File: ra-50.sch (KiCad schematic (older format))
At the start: 172 parts, among them J1 Conn_01x07, J2 Conn_01x05, J3 Conn_01x05, J4 Conn_01x12, J5 Conn_01x20, SW1 MX-NoLED, SW10 MX-NoLED, SW11 MX-NoLED, SW12 MX-NoLED, SW13 MX-NoLED, SW14 MX-NoLED, SW14B1 Rotary_Encoder_Switch, SW15 MX-NoLED, SW16 MX-NoLED, SW17 MX-NoLED, SW18 MX-NoLED, SW19 MX-NoLED, SW2 MX-NoLED, SW20 MX-NoLED, SW21 MX-NoLED, SW22 MX-NoLED, SW23 MX-NoLED, SW24 MX-NoLED, SW25 MX-NoLED, SW26 MX-NoLED, SW27 MX-NoLED, SW28 MX-NoLED, SW29 MX-NoLED, SW3 MX-NoLED, SW30 MX-NoLED, SW31 MX-NoLED, SW32 MX-NoLED, SW33 MX-NoLED, SW34 MX-NoLED, SW35 MX-NoLED, SW36 MX-NoLED, SW37 MX-NoLED, SW38 MX-NoLED, SW39 MX-NoLED, SW4 MX-NoLED, SW40 MX-NoLED, SW41 MX-NoLED, SW42 MX-NoLED, SW43 MX-NoLED, SW44 MX-NoLED, SW45 MX-NoLED, SW46 MX-NoLED, SW47 MX-NoLED, SW48 MX-NoLED, SW49 MX-NoLED, SW5 MX-NoLED, SW50 MX-NoLED, SW51 MX-NoLED, SW52 MX-NoLED, SW53 MX-NoLED, SW54 MX-NoLED, SW55 MX-NoLED, SW56 MX-NoLED, SW57 MX-NoLED, SW58 MX-NoLED, SW59 MX-NoLED, SW6 MX-NoLED, SW60 MX-NoLED, SW61 MX-NoLED, SW62 MX-NoLED, SW63 MX-NoLED, SW64 MX-NoLED, SW65 MX-NoLED, SW66 MX-NoLED, SW67 MX-NoLED, SW68 MX-NoLED, SW69 MX-NoLED, SW7 MX-NoLED, SW8 MX-NoLED, SW9 MX-NoLED

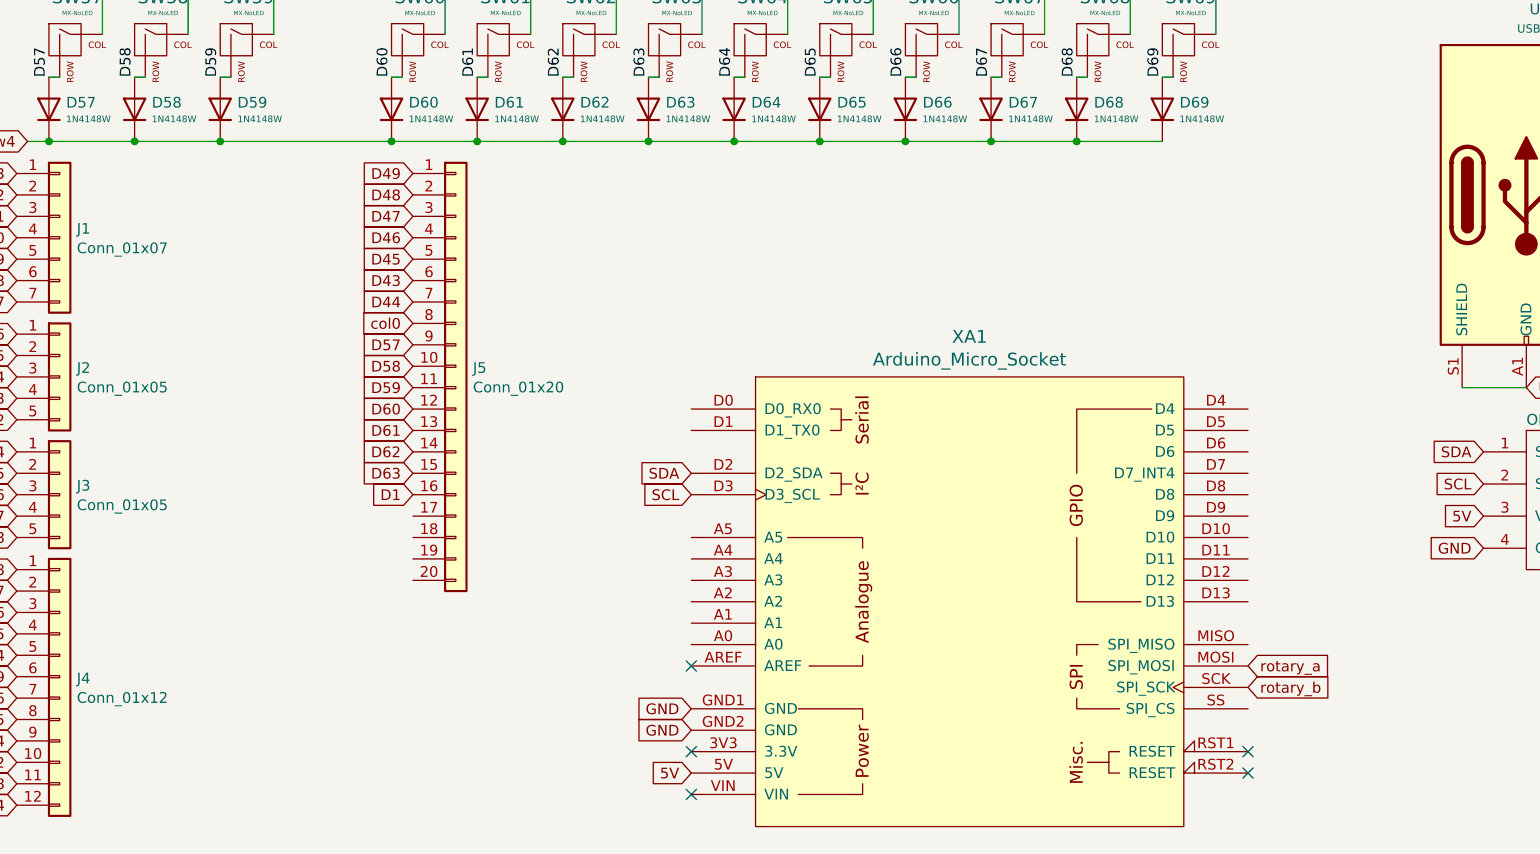
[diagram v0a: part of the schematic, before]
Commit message: update
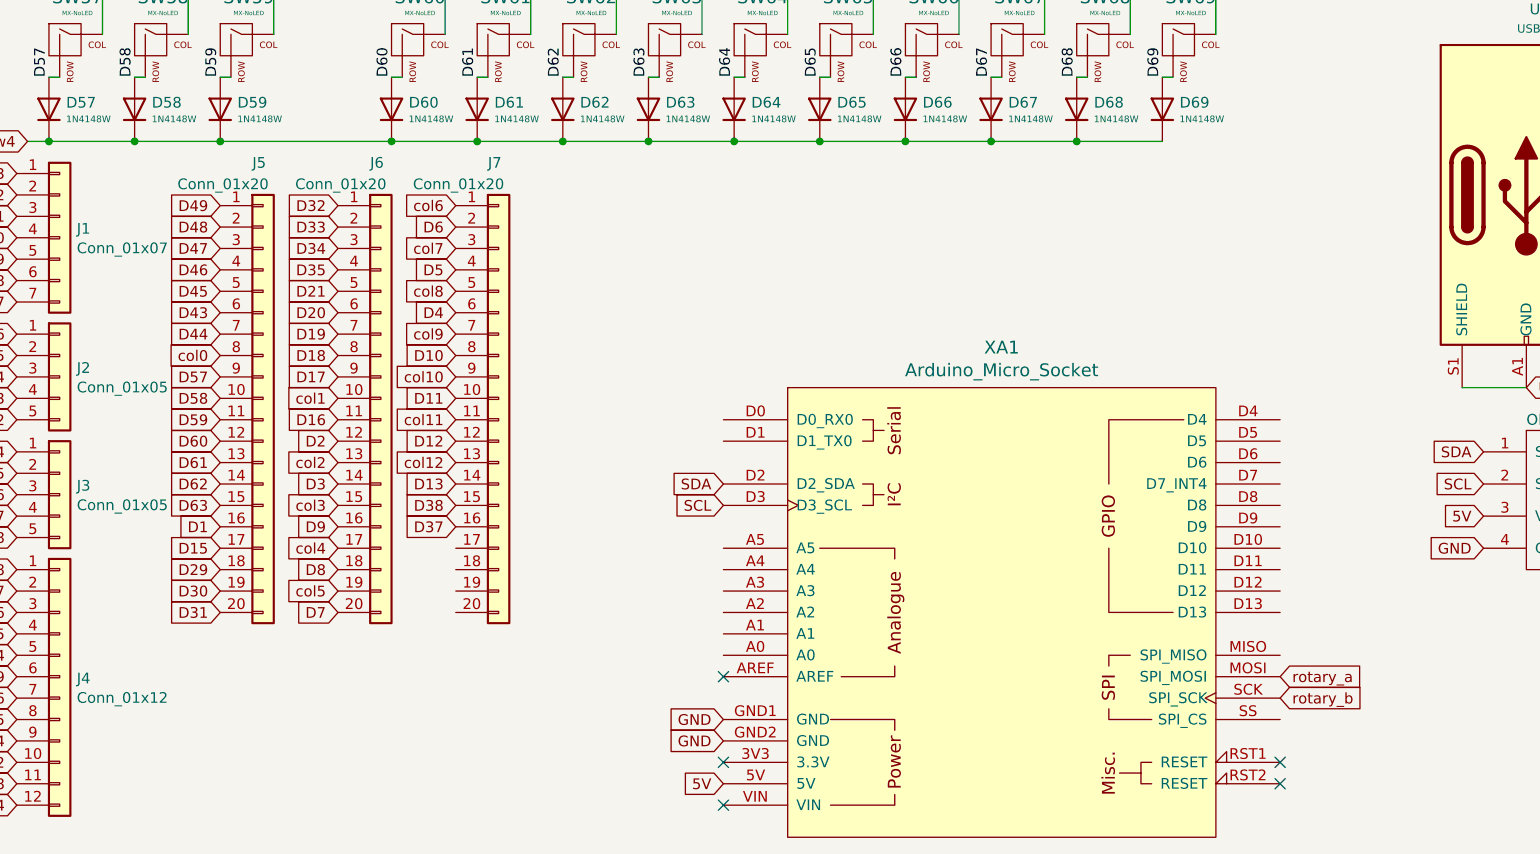
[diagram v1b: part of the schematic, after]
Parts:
- added J6, J7: Conn_01x20, locallib:PinHeader_1x20_via, symbol Connector_Generic:Conn_01x20
- J5: footprint Connector_PinHeader_1.00mm:PinHeader_1x20_P1.00mm_Vertical -> locallib:PinHeader_1x20_via
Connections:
- net D10: now also J7.8 (Pin_8)
- net D11: now also J7.10 (Pin_10)
- net D12: now also J7.12 (Pin_12)
- net D13: now also J7.14 (Pin_14)
- net D15: now also J5.17 (Pin_17)
- net D16: now also J6.11 (Pin_11)
- net D17: now also J6.9 (Pin_9)
- net D18: now also J6.8 (Pin_8)
- net D19: now also J6.7 (Pin_7)
- net D2: now also J6.12 (Pin_12)
- net D20: now also J6.6 (Pin_6)
- net D21: now also J6.5 (Pin_5)
- net D29: now also J5.18 (Pin_18)
- net D3: now also J6.14 (Pin_14)
- net D30: now also J5.19 (Pin_19)
- net D31: now also J5.20 (Pin_20)
- net D32: now also J6.1 (Pin_1)
- net D33: now also J6.2 (Pin_2)
- net D34: now also J6.3 (Pin_3)
- net D35: now also J6.4 (Pin_4)
- net D37: now also J7.16 (Pin_16)
- net D38: now also J7.15 (Pin_15)
- net D4: now also J7.6 (Pin_6)
- net D5: now also J7.4 (Pin_4)
- net D6: now also J7.2 (Pin_2)
- net D7: now also J6.20 (Pin_20)
- net D8: now also J6.18 (Pin_18)
- net D9: now also J6.16 (Pin_16)
- net col1: now also J6.10 (Pin_10)
- net col10: now also J7.9 (Pin_9)
- net col11: now also J7.11 (Pin_11)
- net col12: now also J7.13 (Pin_13)
- net col2: now also J6.13 (Pin_13)
- net col3: now also J6.15 (Pin_15)
- net col4: now also J6.17 (Pin_17)
- net col5: now also J6.19 (Pin_19)
- net col6: now also J7.1 (Pin_1)
- net col7: now also J7.3 (Pin_3)
- net col8: now also J7.5 (Pin_5)
- net col9: now also J7.7 (Pin_7)
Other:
- moved on the sheet: J5, XA1
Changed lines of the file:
@@
 L arduino:Arduino_Micro_Socket XA1
 U 1 1 60EDE630
-P 5150 6650
-F 0 "XA1" H 5150 7887 60  0000 C CNN
-F 1 "Arduino_Micro_Socket" H 5150 7781 60  0000 C CNN
-F 2 "Arduino:Arduino_Micro_Socket" H 6950 10400 60  0001 C CNN
-F 3 "https://store.arduino.cc/arduino-micro" H 6950 10400 60  0001 C CNN
-	1    5150 6650
-	1    0    0    -1
-$EndComp
-Text GLabel 3850 7450 0    50   Input ~ 0
+P 5300 6700
+F 0 "XA1" H 5300 7937 60  0000 C CNN
+F 1 "Arduino_Micro_Socket" H 5300 7831 60  0000 C CNN
+F 2 "Arduino:Arduino_Micro_Socket" H 7100 10450 60  0001 C CNN
+F 3 "https://store.arduino.cc/arduino-micro" H 7100 10450 60  0001 C CNN
+	1    5300 6700
+	1    0    0    -1
+$EndComp
+Text GLabel 4000 7500 0    50   Input ~ 0
 5V
-Text GLabel 3850 7250 0    50   Input ~ 0
+Text GLabel 4000 7300 0    50   Input ~ 0
 GND
-NoConn ~ 3850 7350
-NoConn ~ 3850 7550
-NoConn ~ 3850 6950
-NoConn ~ 6450 7350
-NoConn ~ 6450 7450
+NoConn ~ 4000 7400
+NoConn ~ 4000 7600
+NoConn ~ 4000 7000
+NoConn ~ 6600 7400
+NoConn ~ 6600 7500
 Text GLabel 7550 5950 0    50   Input ~ 0
 SDA
@@
 	-1   0    0    1
 $EndComp
-Text GLabel 3850 7150 0    50   Input ~ 0
+Text GLabel 4000 7200 0    50   Input ~ 0
 GND
 Text GLabel 7250 1200 2    50   Input ~ 0
 GND
-Text GLabel 3850 6150 0    50   Input ~ 0
+Text GLabel 4000 6200 0    50   Input ~ 0
 SCL
-Text GLabel 3850 6050 0    50   Input ~ 0
+Text GLabel 4000 6100 0    50   Input ~ 0
 SDA
-Text GLabel 6450 7050 2    50   Input ~ 0
+Text GLabel 6600 7100 2    50   Input ~ 0
 rotary_b
-Text GLabel 6450 6950 2    50   Input ~ 0
+Text GLabel 6600 7000 2    50   Input ~ 0
 rotary_a
 $Comp
@@
 L Connector_Generic:Conn_01x20 J5
 U 1 1 612D088F
-P 2750 5550
-F 0 "J5" H 2830 5542 50  0000 L CNN
-F 1 "Conn_01x20" H 2830 5451 50  0000 L CNN
-F 2 "Connector_PinHeader_1.00mm:PinHeader_1x20_P1.00mm_Vertical" H 2750 5550 50  0001 C CNN
-F 3 "~" H 2750 5550 50  0001 C CNN
-	1    2750 5550
+P 1850 5700
+F 0 "J5" H 1800 6800 50  0000 L CNN
+F 1 "Conn_01x20" H 1450 6700 50  0000 L CNN
+F 2 "locallib:PinHeader_1x20_via" H 1850 5700 50  0001 C CNN
+F 3 "~" H 1850 5700 50  0001 C CNN
+	1    1850 5700
 	1    0    0    -1
 $EndComp
@@
 Text Label 5650 2700 1    50   ~ 0
 D41
-Text GLabel 2550 4650 0    50   Input ~ 0
+Text GLabel 1650 4800 0    50   Input ~ 0
 D49
-Text GLabel 2550 4750 0    50   Input ~ 0
+Text GLabel 1650 4900 0    50   Input ~ 0
 D48
-Text GLabel 2550 4850 0    50   Input ~ 0
+Text GLabel 1650 5000 0    50   Input ~ 0
 D47
-Text GLabel 2550 4950 0    50   Input ~ 0
+Text GLabel 1650 5100 0    50   Input ~ 0
 D46
-Text GLabel 2550 5050 0    50   Input ~ 0
+Text GLabel 1650 5200 0    50   Input ~ 0
 D45
-Text GLabel 2550 5150 0    50   Input ~ 0
+Text GLabel 1650 5300 0    50   Input ~ 0
 D43
-Text GLabel 2550 5250 0    50   Input ~ 0
+Text GLabel 1650 5400 0    50   Input ~ 0
 D44
-Text GLabel 2550 6050 0    50   Input ~ 0
+Text GLabel 1650 6200 0    50   Input ~ 0
 D63
-Text GLabel 2550 5950 0    50   Input ~ 0
+Text GLabel 1650 6100 0    50   Input ~ 0
 D62
-Text GLabel 2550 5850 0    50   Input ~ 0
+Text GLabel 1650 6000 0    50   Input ~ 0
 D61
-Text GLabel 2550 5750 0    50   Input ~ 0
+Text GLabel 1650 5900 0    50   Input ~ 0
 D60
-Text GLabel 2550 5650 0    50   Input ~ 0
+Text GLabel 1650 5800 0    50   Input ~ 0
 D59
-Text GLabel 2550 5550 0    50   Input ~ 0
+Text GLabel 1650 5700 0    50   Input ~ 0
 D58
-Text GLabel 2550 5450 0    50   Input ~ 0
+Text GLabel 1650 5600 0    50   Input ~ 0
 D57
-Text GLabel 2550 5350 0    50   Input ~ 0
+Text GLabel 1650 5500 0    50   Input ~ 0
 col0
-Text GLabel 2550 6150 0    50   Input ~ 0
+Text GLabel 1650 6300 0    50   Input ~ 0
 D1
 $Comp
@@
 	1    0    0    -1
 $EndComp
+Text GLabel 1650 6400 0    50   Input ~ 0
+D15
+Text GLabel 1650 6500 0    50   Input ~ 0
+D29
+Text GLabel 1650 6600 0    50   Input ~ 0
+D30
+Text GLabel 2200 5700 0    50   Input ~ 0
+col1
+Text GLabel 1650 6700 0    50   Input ~ 0
+D31
+Text GLabel 2200 4800 0    50   Input ~ 0
+D32
+Text GLabel 2200 4900 0    50   Input ~ 0
+D33
+Text GLabel 2200 5000 0    50   Input ~ 0
+D34
+Text GLabel 2200 5100 0    50   Input ~ 0
+D35
+Text GLabel 2200 5200 0    50   Input ~ 0
+D21
+Text GLabel 2200 5300 0    50   Input ~ 0
+D20
+Text GLabel 2200 5400 0    50   Input ~ 0
+D19
+Text GLabel 2200 5500 0    50   Input ~ 0
+D18
+Text GLabel 2200 5600 0    50   Input ~ 0
+D17
+Text GLabel 2200 5800 0    50   Input ~ 0
+D16
+Text GLabel 2200 5900 0    50   Input ~ 0
+D2
+Text GLabel 2200 6000 0    50   Input ~ 0
+col2
+Text GLabel 2200 6100 0    50   Input ~ 0
+D3
+Text GLabel 2750 5700 0    50   Input ~ 0
+D11
+Text GLabel 2750 5900 0    50   Input ~ 0
+D12
+Text GLabel 2750 6100 0    50   Input ~ 0
+D13
+Text GLabel 2200 6200 0    50   Input ~ 0
+col3
+Text GLabel 2200 6400 0    50   Input ~ 0
+col4
+Text GLabel 2750 5500 0    50   Input ~ 0
+D10
+$Comp
+L Connector_Generic:Conn_01x20 J6
+U 1 1 60F7AB70
+P 2400 5700
+F 0 "J6" H 2350 6800 50  0000 L CNN
+F 1 "Conn_01x20" H 2000 6700 50  0000 L CNN
+F 2 "locallib:PinHeader_1x20_via" H 2400 5700 50  0001 C CNN
+F 3 "~" H 2400 5700 50  0001 C CNN
+	1    2400 5700
+	1    0    0    -1
+$EndComp
+Text GLabel 2200 6600 0    50   Input ~ 0
+col5
+Text GLabel 2750 4800 0    50   Input ~ 0
+col6
+Text GLabel 2750 5000 0    50   Input ~ 0
+col7
+Text GLabel 2750 5200 0    50   Input ~ 0
+col8
+Text GLabel 2750 5400 0    50   Input ~ 0
+col9
+Text GLabel 2750 5600 0    50   Input ~ 0
+col10
+Text GLabel 2750 5800 0    50   Input ~ 0
+col11
+Text GLabel 2750 6000 0    50   Input ~ 0
+col12
+Text GLabel 2750 6200 0    50   Input ~ 0
+D38
+Text GLabel 2200 6700 0    50   Input ~ 0
+D7
+Text GLabel 2200 6500 0    50   Input ~ 0
+D8
+Text GLabel 2750 4900 0    50   Input ~ 0
+D6
+Text GLabel 2750 5100 0    50   Input ~ 0
+D5
+Text GLabel 2750 5300 0    50   Input ~ 0
+D4
+Text GLabel 2200 6300 0    50   Input ~ 0
+D9
+$Comp
+L Connector_Generic:Conn_01x20 J7
+U 1 1 6115908E
+P 2950 5700
+F 0 "J7" H 2900 6800 50  0000 L CNN
+F 1 "Conn_01x20" H 2550 6700 50  0000 L CNN
+F 2 "locallib:PinHeader_1x20_via" H 2950 5700 50  0001 C CNN
+F 3 "~" H 2950 5700 50  0001 C CNN
+	1    2950 5700
+	1    0    0    -1
+$EndComp
+Text GLabel 2750 6300 0    50   Input ~ 0
+D37
 $EndSCHEMATC

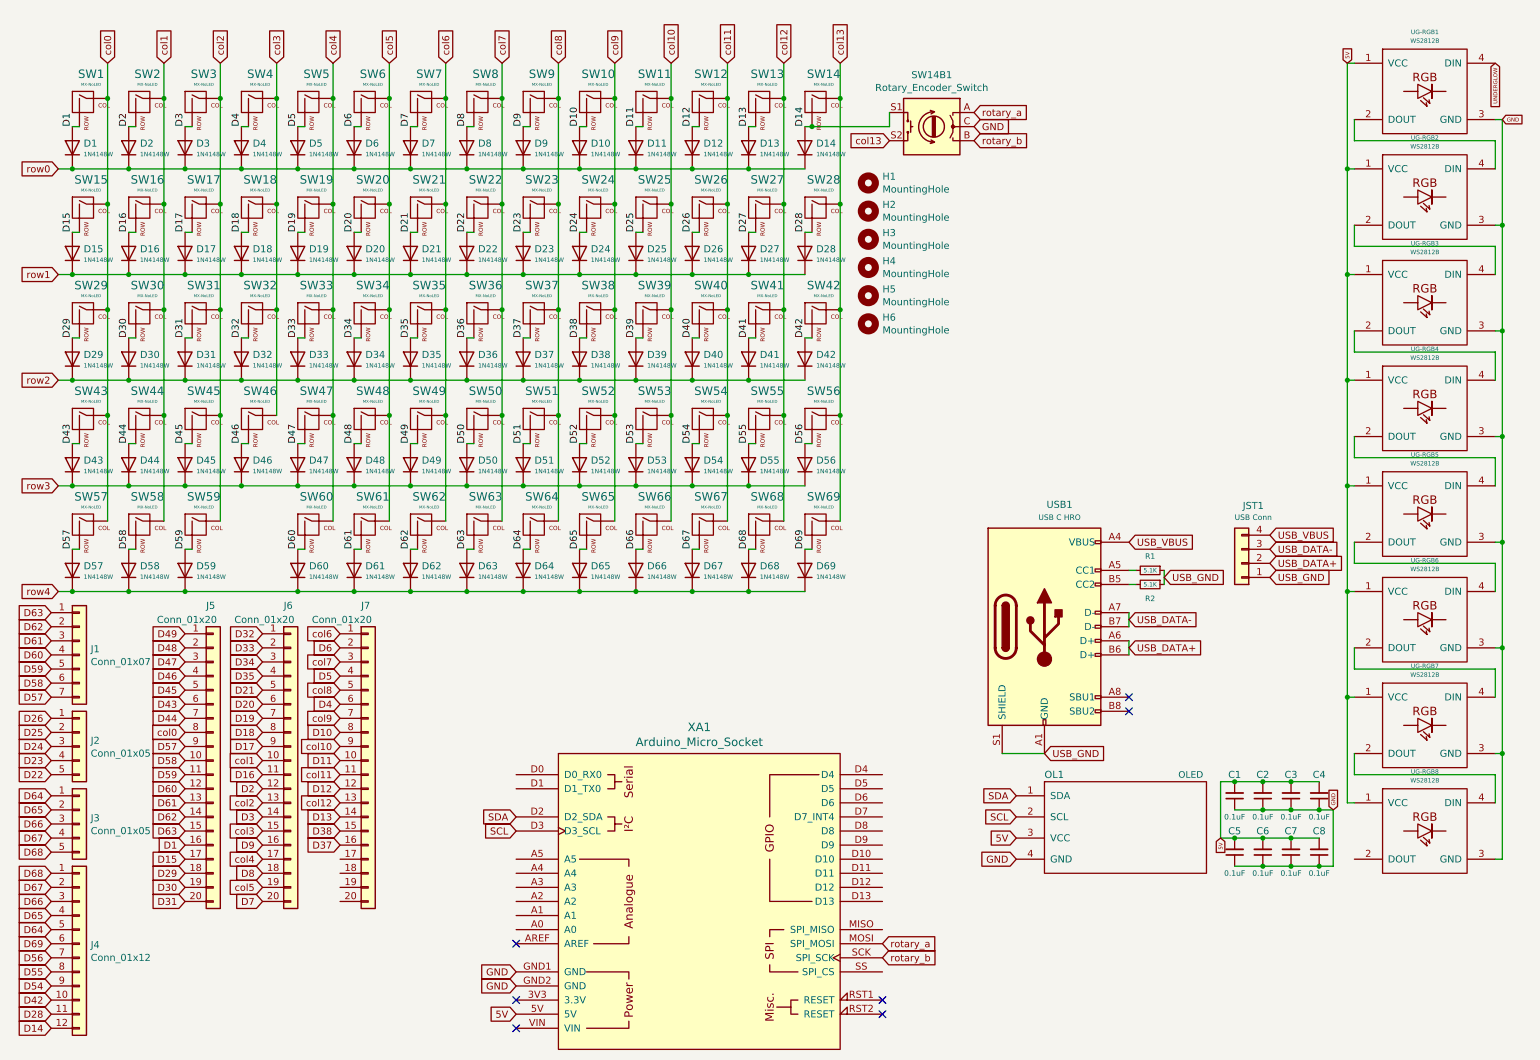
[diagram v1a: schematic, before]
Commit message: big revision
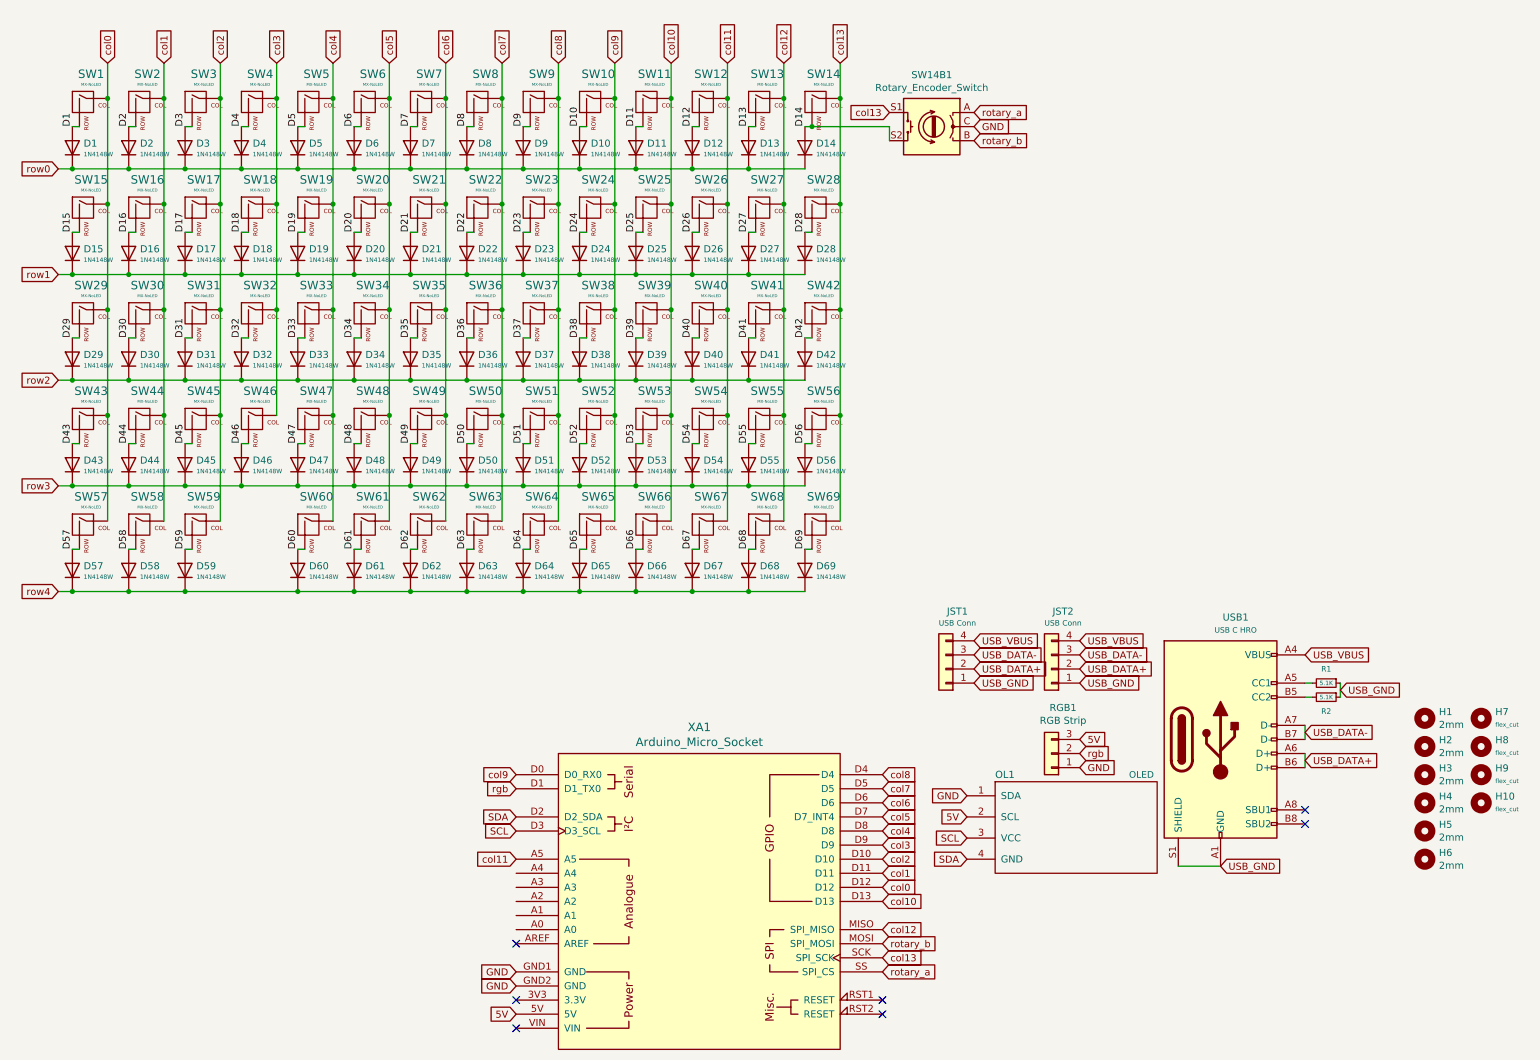
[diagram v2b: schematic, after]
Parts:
- removed C1, C2, C3, C4, C5, C6, C7, C8: 0.1uF, Capacitor_SMD:C_0201_0603Metric_Pad0.64x0.40mm_HandSolder, symbol Device:C_Small
- removed J1: Conn_01x07, Connector_PinHeader_1.00mm:PinHeader_1x07_P1.00mm_Vertical, symbol Connector_Generic:Conn_01x07
- removed J2, J3: Conn_01x05, Connector_PinHeader_1.00mm:PinHeader_1x05_P1.00mm_Vertical, symbol Connector_Generic:Conn_01x05
- removed J4: Conn_01x12, Connector_PinHeader_1.00mm:PinHeader_1x12_P1.00mm_Vertical, symbol Connector_Generic:Conn_01x12
- removed J5, J6, J7: Conn_01x20, locallib:PinHeader_1x20_via, symbol Connector_Generic:Conn_01x20
- removed UG-RGB1, UG-RGB2, UG-RGB3, UG-RGB4, UG-RGB5, UG-RGB6, UG-RGB7, UG-RGB8: WS2812B, LED_SMD:LED_WS2812B_PLCC4_5.0x5.0mm_P3.2mm, symbol ws2812b:WS2812B
- added H10, H7, H8, H9: flex_cut, locallib:LongOvalCut_225mmFlexCut, symbol Mechanical:MountingHole
- added JST2: USB Conn, Connector_JST:JST_GH_SM04B-GHS-TB_1x04-1MP_P1.25mm_Horizontal, symbol Connector_Generic:Conn_01x04
- added RGB1: RGB Strip, Connector_PinSocket_2.54mm:PinSocket_1x03_P2.54mm_Vertical, symbol Connector_Generic:Conn_01x03
- D1, D10, D11, D12, D13, D14, D15, D16, D17, D18, D19, D2, D20, D21, D22, D23, D24, D25, D26, D27, D28, D29, D3, D30, D31, D32, D33, D34, D35, D36, D37, D38, D39, D4, D40, D41, D42, D43, D44, D45, D46, D47, D48, D49, D5, D50, D51, D52, D53, D54, D55, D56, D57, D58, D59, D6, D60, D61, D62, D63, D64, D65, D66, D67, D68, D69, D7, D8, D9: footprint Keebio-Parts:D_SOD123 -> master-Keebio-Parts:D_SOD123
- H1, H2, H3, H4, H5, H6: value MountingHole -> 2mm
- JST1: footprint Connector_JST:JST_GH_SM04B-GHS-TB_1x04-1MP_P1.25mm_Horizontal -> Connector_PinHeader_2.54mm:PinHeader_1x04_P2.54mm_Vertical
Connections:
- net 5V: now also OL1.2 (SCL), RGB1.3 (Pin_3); no longer OL1.3 (VCC)
- net D14: now also SW14B1.S2; no longer SW14B1.S1
- net GND: now also OL1.1 (SDA), RGB1.1 (Pin_1); no longer OL1.4 (GND)
- net SCL: now also OL1.3 (VCC); no longer OL1.2 (SCL)
- net SDA: now also OL1.4 (GND); no longer OL1.1 (SDA)
- net USB_DATA+: now also JST2.2 (Pin_2)
- net USB_DATA-: now also JST2.3 (Pin_3)
- net USB_GND: now also JST2.1 (Pin_1)
- net USB_VBUS: now also JST2.4 (Pin_4)
- net col0: now also XA1.D12
- net col1: now also XA1.D11
- net col10: now also XA1.D13
- net col11: now also XA1.A5
- net col12: now also XA1.MISO (SPI_MISO)
- net col13: now also SW14B1.S1, XA1.SCK (SPI_SCK); no longer SW14B1.S2
- net col2: now also XA1.D10
- net col3: now also XA1.D9
- net col4: now also XA1.D8
- net col5: now also XA1.D7 (D7_INT4)
- net col6: now also XA1.D6
- net col7: now also XA1.D5
- net col8: now also XA1.D4
- net col9: now also XA1.D0 (D0_RX0)
- net rotary_a: now also XA1.SS (SPI_CS); no longer XA1.MOSI (SPI_MOSI)
- net rotary_b: now also XA1.MOSI (SPI_MOSI); no longer XA1.SCK (SPI_SCK)
- net rgb: now reaches XA1.D1 (D1_TX0)
- net rgb: now also RGB1.2 (Pin_2)
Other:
- moved on the sheet: H1, H2, H3, H4, H5, H6, OL1, R1, R2, USB1
